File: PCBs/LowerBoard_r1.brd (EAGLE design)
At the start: 93 x 57.7 mm, 14 parts, among them K1 G2R2, P1 HEADER_5X2, Q1 2N7000

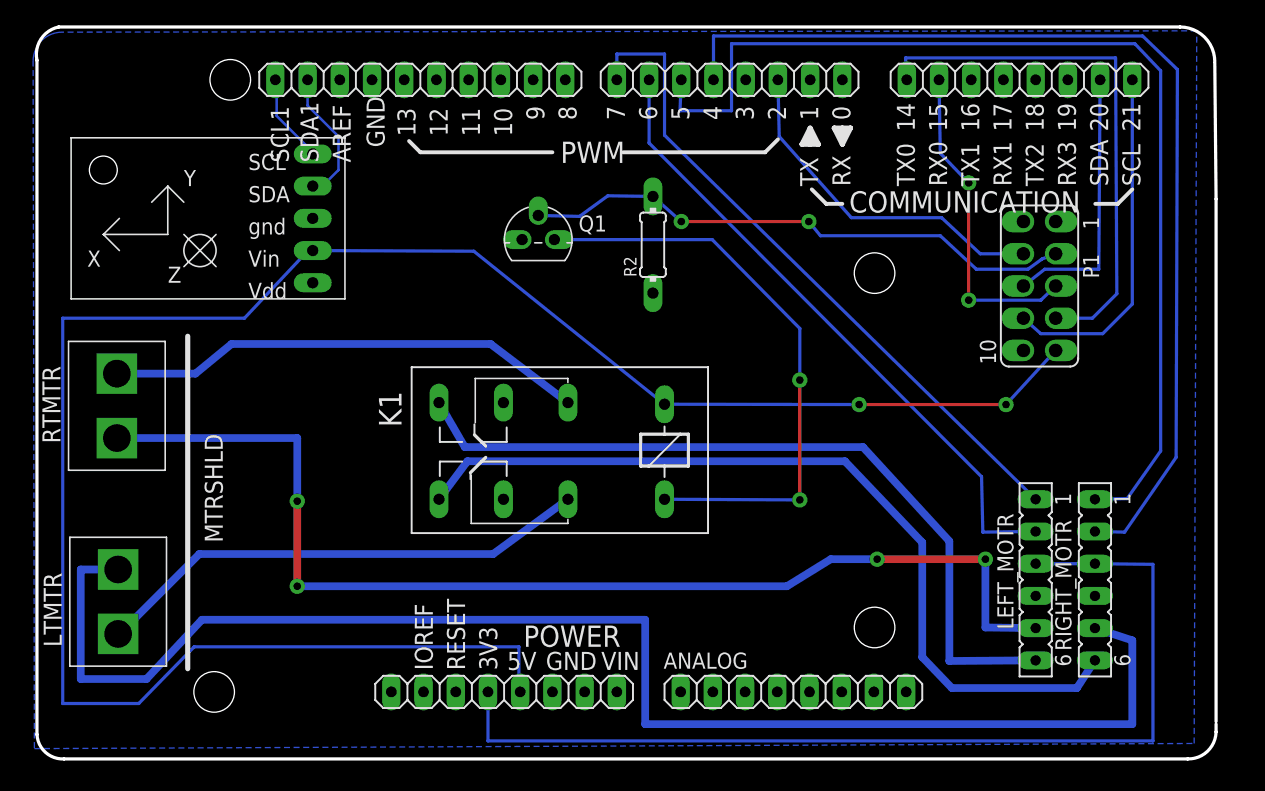
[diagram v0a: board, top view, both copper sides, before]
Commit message: finished eagle file for lower PCB
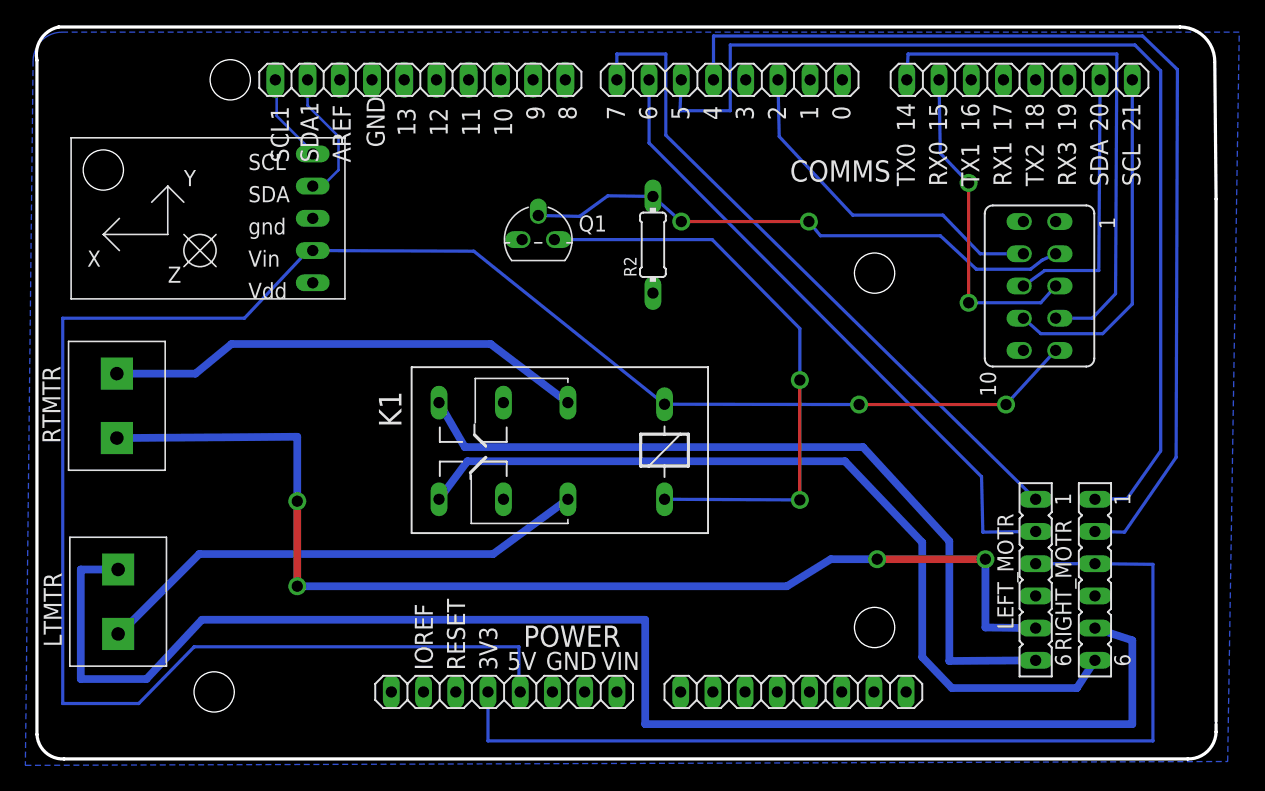
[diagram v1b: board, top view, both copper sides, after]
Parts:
- removed COMMUNICATION: 8x1F-H8.5, SmartPrj:1X08
- added COMMS: (no value), LowerBoard_r1:1X08
- added DRILEGEND: (no value), drilegend:DRILEGEND
- ANALOG, POWER, PWML: device SmartPrj:1X08 -> LowerBoard_r1:1X08
- LEFT_MOTR, RIGHT_MOTR: device con-lsta:FE06 -> LowerBoard_r1:FE06
- P1: device myDevices:HEADER_5X2 -> LowerBoard_r1:HEADER_5X2
- PWMH: device SmartPrj:1X10 -> LowerBoard_r1:1X10
- U$11, U$12: device myDevices:TB2_PKG -> LowerBoard_r1:TB2_PKG
- U$5: device myDevices:POLOLU_IMU9V2 -> LowerBoard_r1:POLOLU_IMU9V2
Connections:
- net SCL0: now also COMMS.8; no longer COMMUNICATION.8
- net SDA0: now also COMMS.7; no longer COMMUNICATION.7
- net XBEE_DIN: now also COMMS.1; no longer COMMUNICATION.1
- net XBEE_DOUT: now also COMMS.2; no longer COMMUNICATION.2
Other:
- board text added: "01-16"
- board text added: "01-20"
- board text added: "LAYER-STACK"
- board text removed: "MTRSHLD"
- board text removed: "PC1"
- board text removed: "PC2"
- board text removed: "PWM"
- board text removed: "RX"
- board text removed: "TX"
